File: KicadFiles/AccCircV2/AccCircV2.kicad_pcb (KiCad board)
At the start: 2 copper layers, 58.7 x 33.2 mm, 13 parts, among them J1 AccelConnector, J2 ADCInput, J3 IO, J4 ExtSupply, U1 MCP602, U2 LM385Z-ADJ

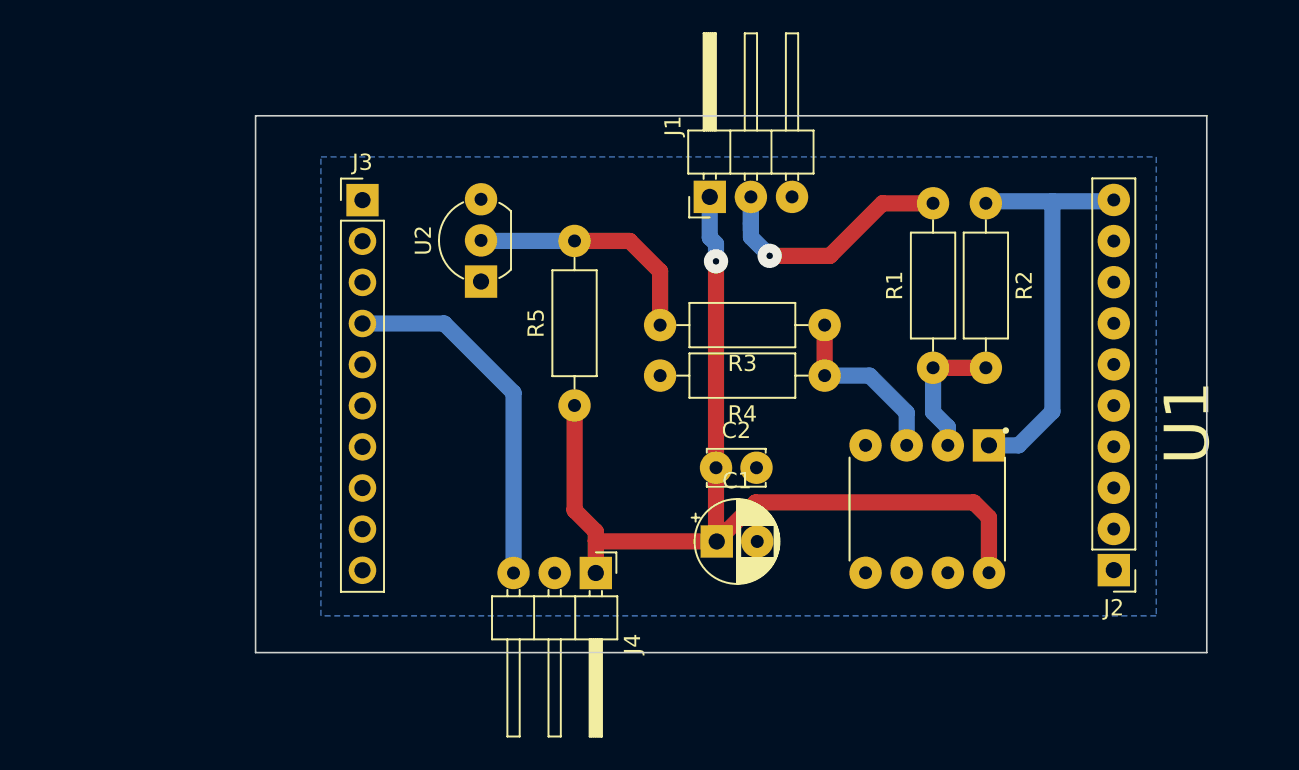
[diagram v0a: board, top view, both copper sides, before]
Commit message: New project CCS
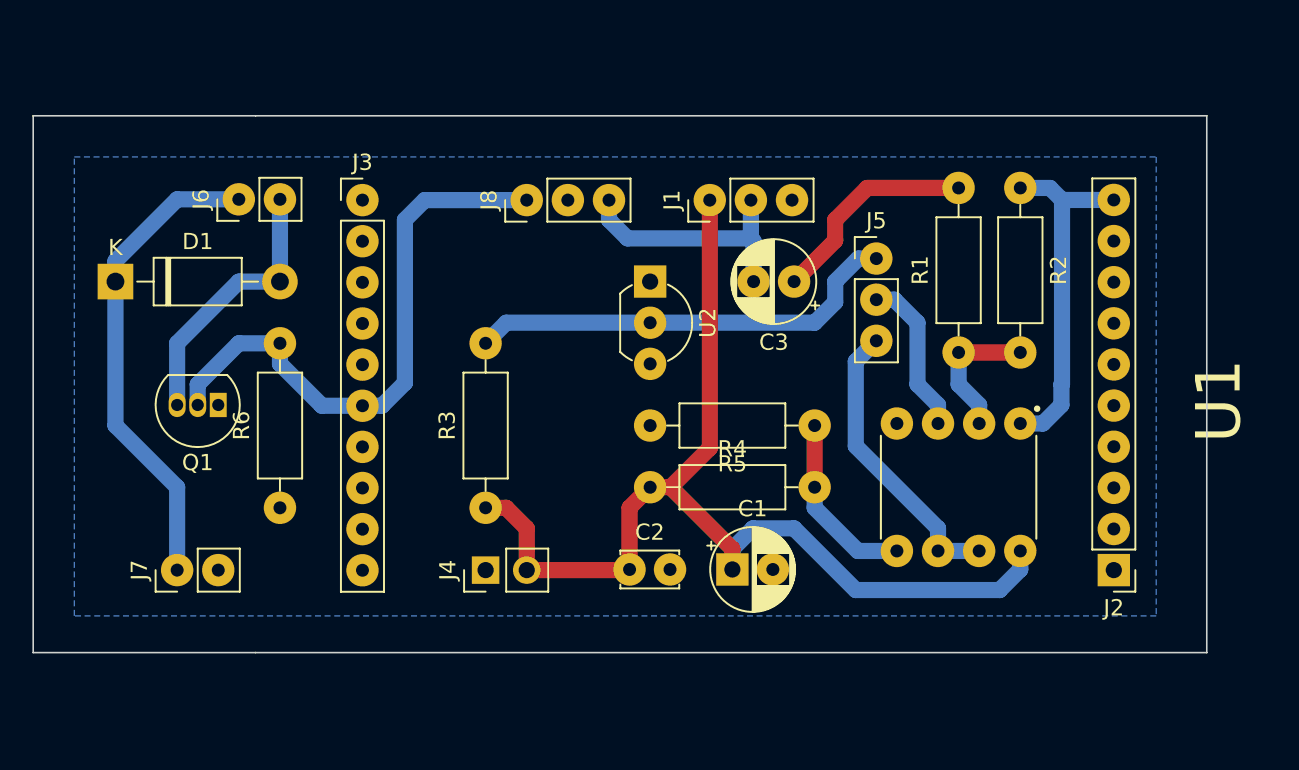
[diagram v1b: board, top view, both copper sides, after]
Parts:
- removed the R3 at (90.8, 33.2)
- added C3: 10uF, Capacitor_THT:CP_Radial_D5.0mm_P2.50mm, F.Cu at (88.9, 30.5)
- added D1: 1N4001, Diode_THT:D_DO-41_SOD81_P10.16mm_Horizontal, F.Cu at (47.0, 30.5)
- added J5: VoltageRefSel, Connector_PinHeader_2.54mm:PinHeader_1x03_P2.54mm_Vertical, F.Cu at (94.0, 29.1)
- added J6: Solenoid Connector, Connector_PinHeader_2.54mm:PinHeader_1x02_P2.54mm_Vertical, F.Cu at (54.6, 25.4)
- added J7: ExternalSupply5V, Connector_PinHeader_2.54mm:PinHeader_1x02_P2.54mm_Vertical, F.Cu at (50.8, 48.3)
- added J8: ControlSig, Connector_PinHeader_2.54mm:PinHeader_1x03_P2.54mm_Vertical, F.Cu at (72.4, 25.4)
- added Q1: TN0207, Package_TO_SOT_THT:TO-92_Inline, F.Cu at (53.3, 38.1)
- added R5: R, Resistor_THT:R_Axial_DIN0207_L6.3mm_D2.5mm_P10.16mm_Horizontal, F.Cu at (90.2, 39.4)
- added R6: 10k, Resistor_THT:R_Axial_DIN0207_L6.3mm_D2.5mm_P10.16mm_Horizontal, F.Cu at (57.1, 44.5)
- J1: footprint Connector_PinHeader_2.54mm:PinHeader_1x03_P2.54mm_Horizontal -> Connector_PinHeader_2.54mm:PinHeader_1x03_P2.54mm_Vertical
- J4: value ExtSupply -> ExternalSupply3V3; footprint Connector_PinHeader_2.54mm:PinHeader_1x03_P2.54mm_Horizontal -> Connector_PinHeader_2.54mm:PinHeader_1x02_P2.54mm_Vertical
- moved R4 12.8 mm to (80.0, 43.2), turned to 0 degrees
- moved U2 10.4 mm to (80.0, 30.5), turned to 270 degrees
- moved R3 8.37 mm to (69.8, 44.5)
- moved C2 8.25 mm to (78.7, 48.3)
- moved J4 6.81 mm to (69.8, 48.3), turned to 90 degrees
- moved U1 2.36 mm to (99.1, 43.2)
- moved R2 2.33 mm to (102.9, 24.7)
- moved C1 1.98 mm to (85.1, 48.3)
- moved R1 1.84 mm to (99.1, 34.9)
- moved J1 0.20 mm to (83.7, 25.4)
- renumbered R5 to R3
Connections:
- C1 pad 1: VDD -> +3V3
- C2 pad 1: VDD -> +3V3
- J1 pad 1: VDD -> +3V3
- J1 pad 2: Net-(J1-Pad2) -> AccSignal
- J2 pad 1: Net-(J2-Pad1) -> (no net)
- J2 pad 2: Net-(J2-Pad2) -> (no net)
- J2 pad 3: Net-(J2-Pad3) -> (no net)
- J2 pad 4: Net-(J2-Pad4) -> (no net)
- J2 pad 5: Net-(J2-Pad5) -> (no net)
- J2 pad 6: Net-(J2-Pad6) -> (no net)
- J2 pad 7: Net-(J2-Pad7) -> (no net)
- J2 pad 8: Net-(J2-Pad8) -> (no net)
- J2 pad 9: Net-(J2-Pad9) -> (no net)
- J3 pad 1: GND -> (no net)
- J3 pad 10: Net-(J3-Pad10) -> GND
- J3 pad 2: Net-(J3-Pad2) -> (no net)
- J3 pad 3: Net-(J3-Pad3) -> (no net)
- J3 pad 4: PIN3.2 -> (no net)
- J3 pad 5: Net-(J3-Pad5) -> (no net)
- J3 pad 6: Net-(J3-Pad6) -> PIN3.2
- J3 pad 7: Net-(J3-Pad7) -> (no net)
- J3 pad 8: Net-(J3-Pad8) -> (no net)
- J3 pad 9: Net-(J3-Pad9) -> (no net)
- J4 pad 1: VDD -> GND
- J4 pad 2: GND -> +3V3
- R1 pad 2: Net-(J1-Pad2) -> Net-(C3-Pad1)
- R3 pad 1: VDD -> +3V3
- R4 pad 1: Net-(R3-Pad1) -> +3V3
- R4 pad 2: GND -> Net-(R4-Pad2)
- U1 pad 3: Net-(R3-Pad1) -> Net-(J5-Pad2)
- U1 pad 5: (no net) -> Net-(R4-Pad2)
- U1 pad 6: (no net) -> VolDivider
- U1 pad 7: (no net) -> VolDivider
- U1 pad 8: VDD -> +3V3
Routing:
- net +3V3: track 0.00 -> 67.1 mm
- net VDD: track 61.5 -> 0.00 mm, vias 1 -> 0
- net +5V: track 0.00 -> 29.9 mm
- net VolDivider: track 0.00 -> 18.1 mm
- net Net-(J1-Pad2): track 17.6 -> 0.00 mm, vias 1 -> 0
- net Net-(D1-Pad2): track 0.00 -> 16.8 mm
- net AccSignal: track 0.00 -> 15.6 mm
- net PIN3.2: track 22.5 -> 36.1 mm
- net Net-(C3-Pad1): track 0.00 -> 13.3 mm
- net VolRef1V2: track 15.2 -> 27.0 mm
- net Net-(R4-Pad2): track 0.00 -> 11.3 mm
- net Net-(R3-Pad1): track 11.2 -> 0.00 mm
- net Net-(J5-Pad2): track 0.00 -> 9.88 mm
- net Net-(J2-Pad10): track 26.0 -> 22.2 mm
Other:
- board size 58.7 x 33.2 mm -> 72.5 x 33.2 mm
